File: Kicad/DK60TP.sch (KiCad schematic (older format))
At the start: 19 parts, among them J1 USB_mini_micro_B, M1 MISC, M2 MISC, P1 MOUSE_BOARD, SW1 SW_PUSH, U0 ATMEGA32U4-MU, X1 XTAL_GND

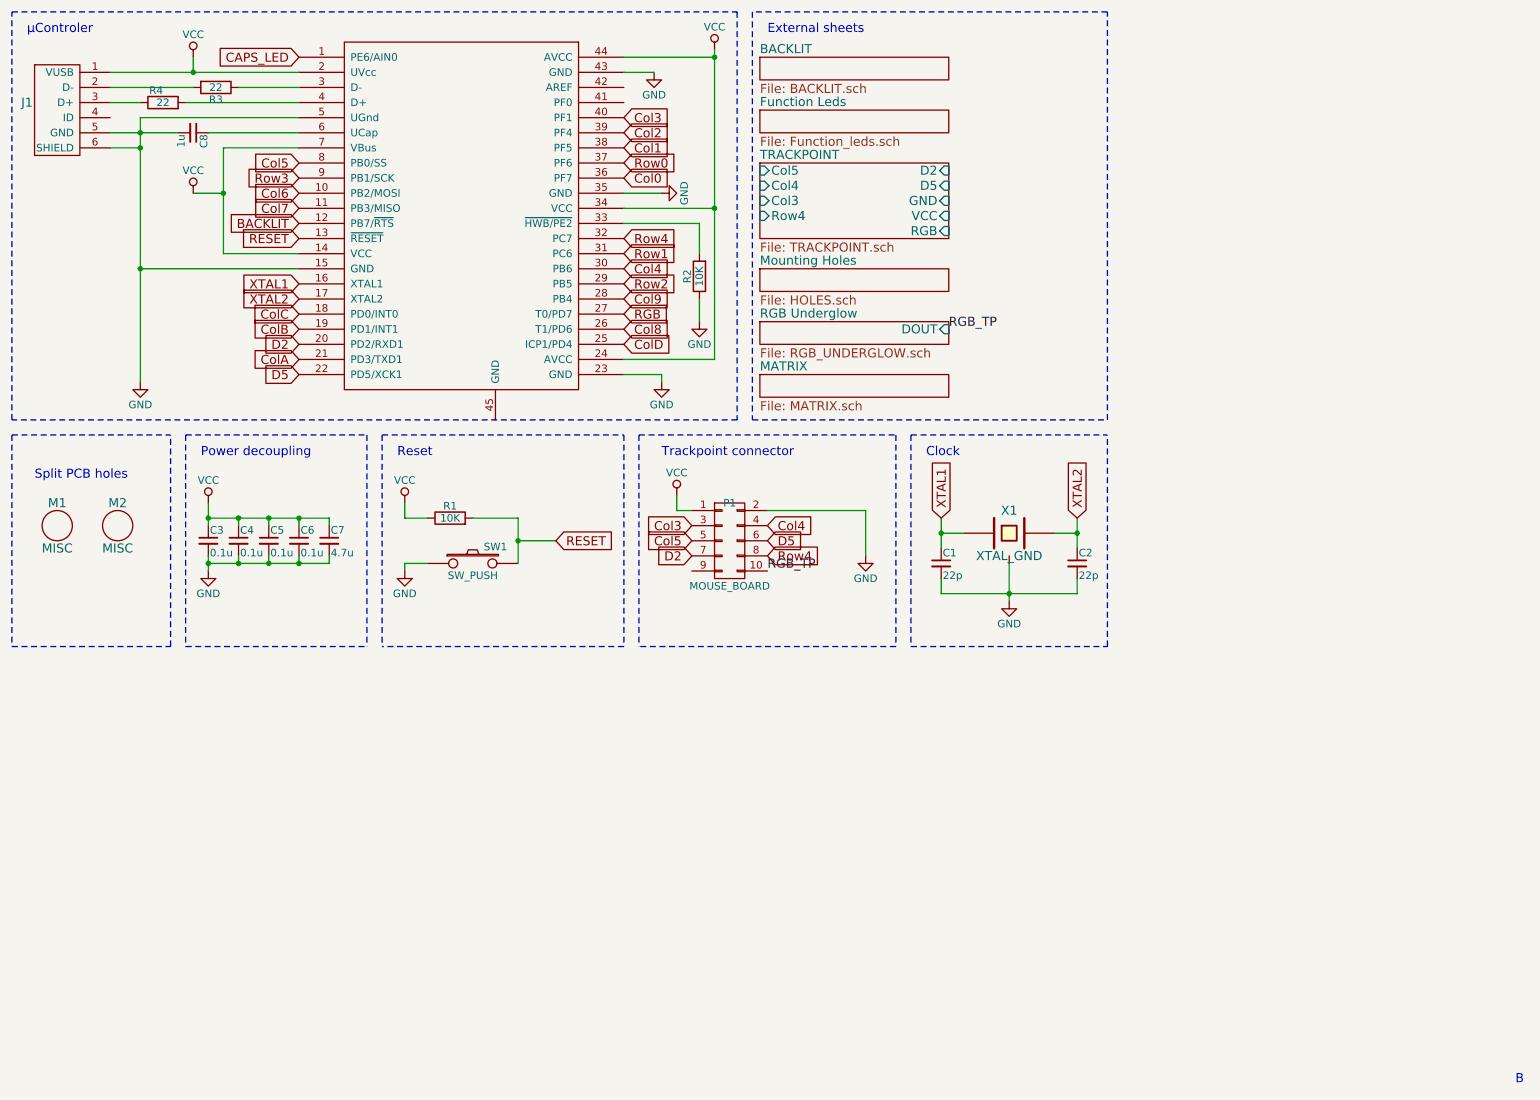
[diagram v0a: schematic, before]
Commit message: - Updated ATMEGA to MU version
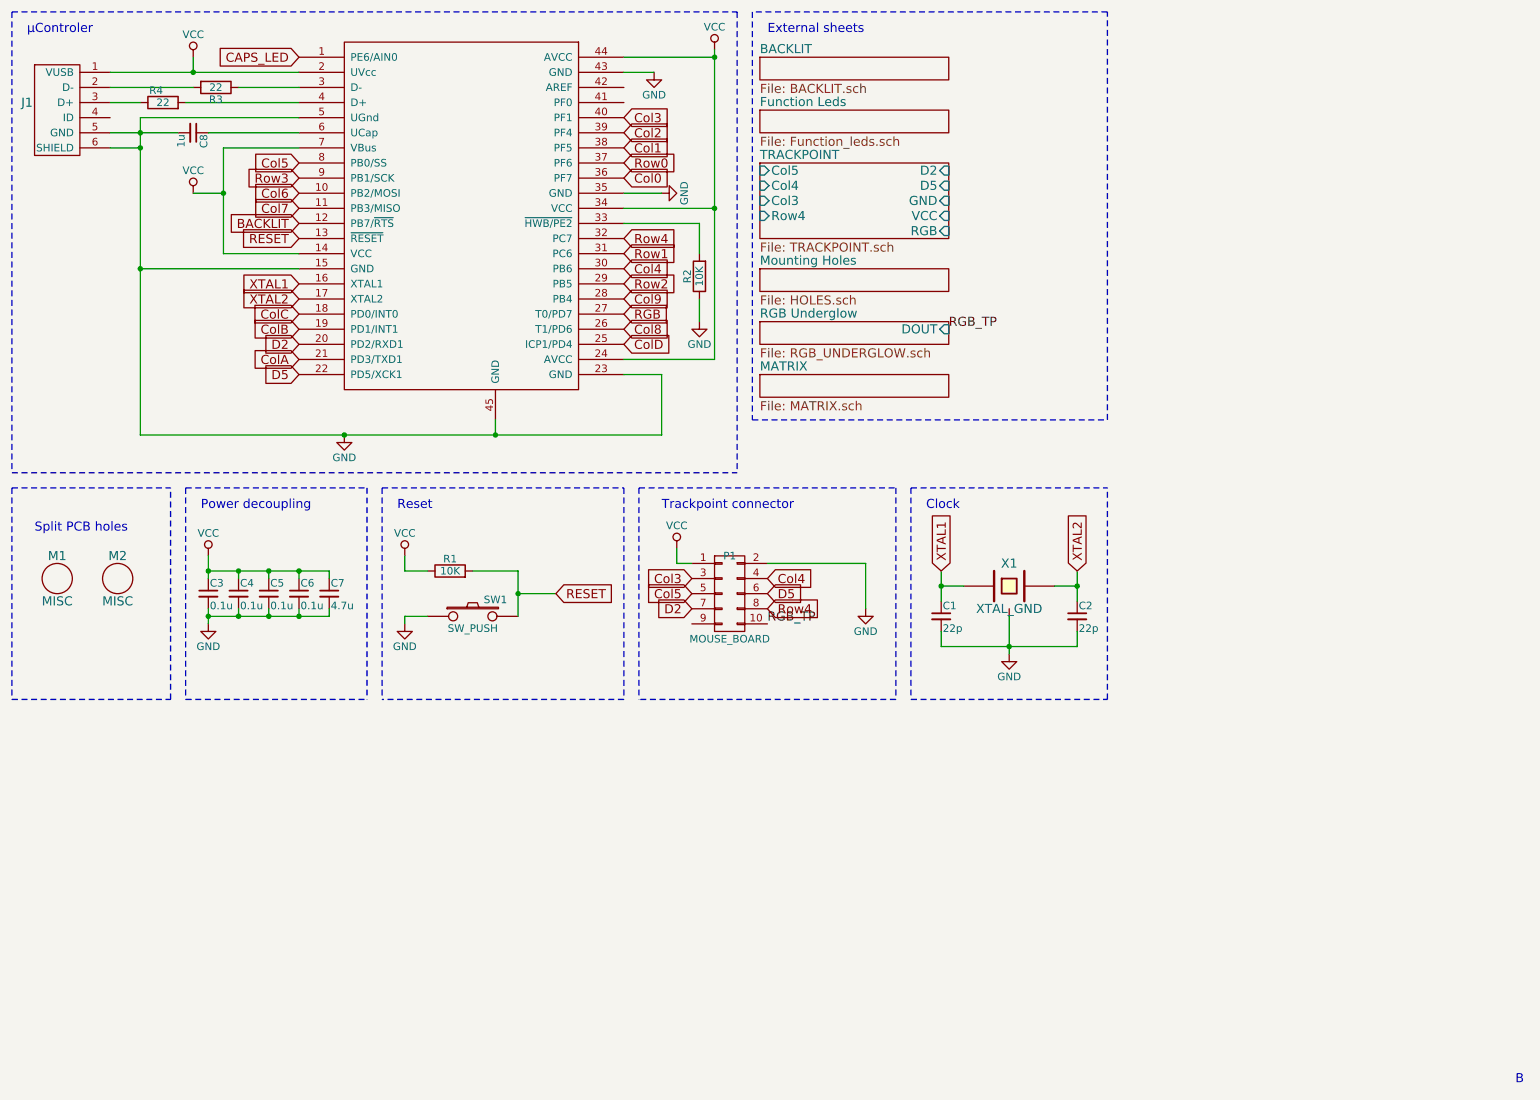
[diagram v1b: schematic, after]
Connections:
- net GND: now also U0.45 (GND)
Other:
- moved on the sheet: C1, C2, C3, C4, C5, C6, C7, M1, M2, P1, R1, SW1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

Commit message: - Updated ATMEGA controller (AU and MU package)
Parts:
- U0: symbol ATMEGA32U4 -> ATMEGA32U4-MU
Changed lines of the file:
@@
 EESchema Schematic File Version 2
 LIBS:power
-LIBS:device
-LIBS:transistors
-LIBS:conn
-LIBS:linear
-LIBS:regul
-LIBS:74xx
-LIBS:cmos4000
-LIBS:adc-dac
-LIBS:memory
-LIBS:xilinx
-LIBS:microcontrollers
-LIBS:dsp
-LIBS:microchip
-LIBS:analog_switches
-LIBS:motorola
-LIBS:texas
-LIBS:intel
-LIBS:audio
-LIBS:interface
-LIBS:digital-audio
-LIBS:philips
-LIBS:display
-LIBS:cypress
-LIBS:siliconi
-LIBS:opto
-LIBS:atmel
-LIBS:contrib
-LIBS:valves
-LIBS:keyboard_parts
-LIBS:mkl27z256vfm4
-LIBS:TS65
 LIBS:DK60TP-cache
 EELAYER 25 0
@@
 $EndComp
 $Comp
-L ATMEGA32U4 U0
+L ATMEGA32U4-MU U0
 U 1 1 591F6C9B
 P 3550 1900

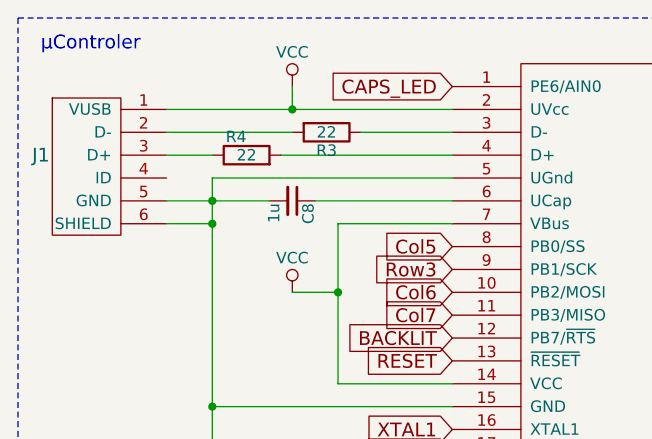
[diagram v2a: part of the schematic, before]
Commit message: - Simplifying routage (1 over n)
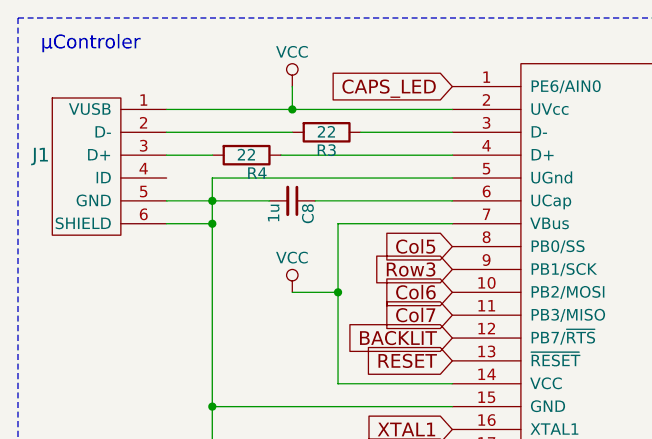
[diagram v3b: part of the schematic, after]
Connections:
- net at U0.4 (D+): now also R4.1; no longer R4.2
- net at J1.3 (D+): now also R4.2; no longer R4.1
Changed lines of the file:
@@
 F 3 "" H 1600 1150 50  0001 C CNN
 	1    1600 1150
-	0    -1   -1   0
+	0    1    1    0
 $EndComp
 $Comp

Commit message: - Simplifying routing (3/n)
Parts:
- M1, M2: footprint Footprint:BreakHoles -> Footprint:BreakHoles_small
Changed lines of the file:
@@
 F 0 "M1" H 900 4450 60  0000 C CNN
 F 1 "MISC" H 900 4150 60  0000 C CNN
-F 2 "Footprint:BreakHoles" H 900 4300 60  0001 C CNN
+F 2 "Footprint:BreakHoles_small" H 900 4300 60  0001 C CNN
 F 3 "" H 900 4300 60  0000 C CNN
 	1    900  4300
@@
 F 0 "M2" H 1300 4450 60  0000 C CNN
 F 1 "MISC" H 1300 4150 60  0000 C CNN
-F 2 "Footprint:BreakHoles" H 1300 4300 60  0001 C CNN
+F 2 "Footprint:BreakHoles_small" H 1300 4300 60  0001 C CNN
 F 3 "" H 1300 4300 60  0000 C CNN
 	1    1300 4300
